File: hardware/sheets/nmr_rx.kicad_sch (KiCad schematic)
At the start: 94 parts, among them J3 C2937625_-_Conn_01x03, J9 C2937625_-_Conn_01x03, U701 SI5351A-B-GT, U702 74HC74D,653, U703 OPA1656IDR, U704 DG419DY-T1-E3, U705 OPA1612AIDR, U706 OPA1612AIDR, U901 TS5A23157DGSR, U902 TS5A23157DGSR, Y701 25 MHz

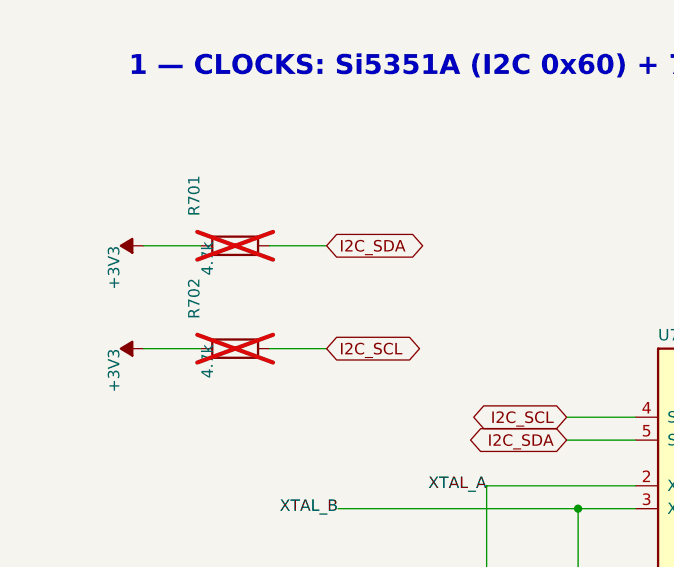
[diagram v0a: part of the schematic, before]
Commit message: hardware: board, sheets and DC jack footprint as on disk 2026-09-27 (snapshot committed by the projector-developer session, Shayne 2026-09-27)
Co-Authored-By: Claude Fable 5.1 <noreply@anthropic.com>
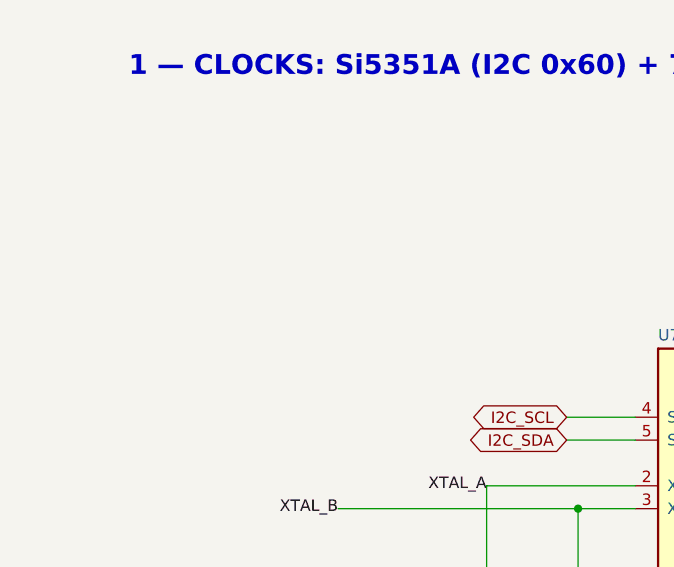
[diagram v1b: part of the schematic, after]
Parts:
- removed R701, R702: 4.7k, Resistor_SMD:R_0603_1608Metric, symbol class_board:R0603_4R7k
